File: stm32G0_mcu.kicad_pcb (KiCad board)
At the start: 4 copper layers, 70 x 45 mm, 54 parts, among them J1 Conn_01x04_Pin, J2 Conn_01x06_Pin, J3 Conn_01x04_Pin, SW1 SW_Nidec_CAS-120A1, SW2 SW_Push, SW3 SW_Push, U1 STM32G0B0KETx, U7 FT230XS

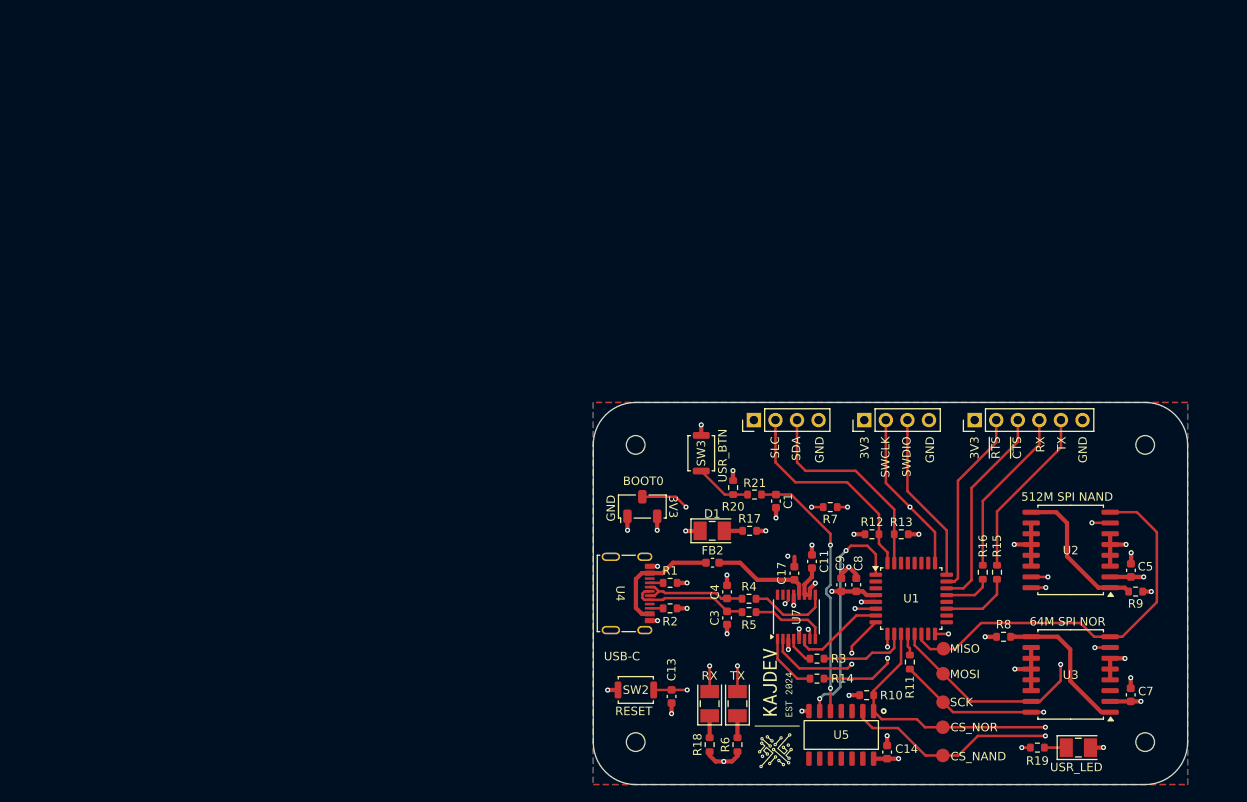
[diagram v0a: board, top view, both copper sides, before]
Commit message: fsdfsdf
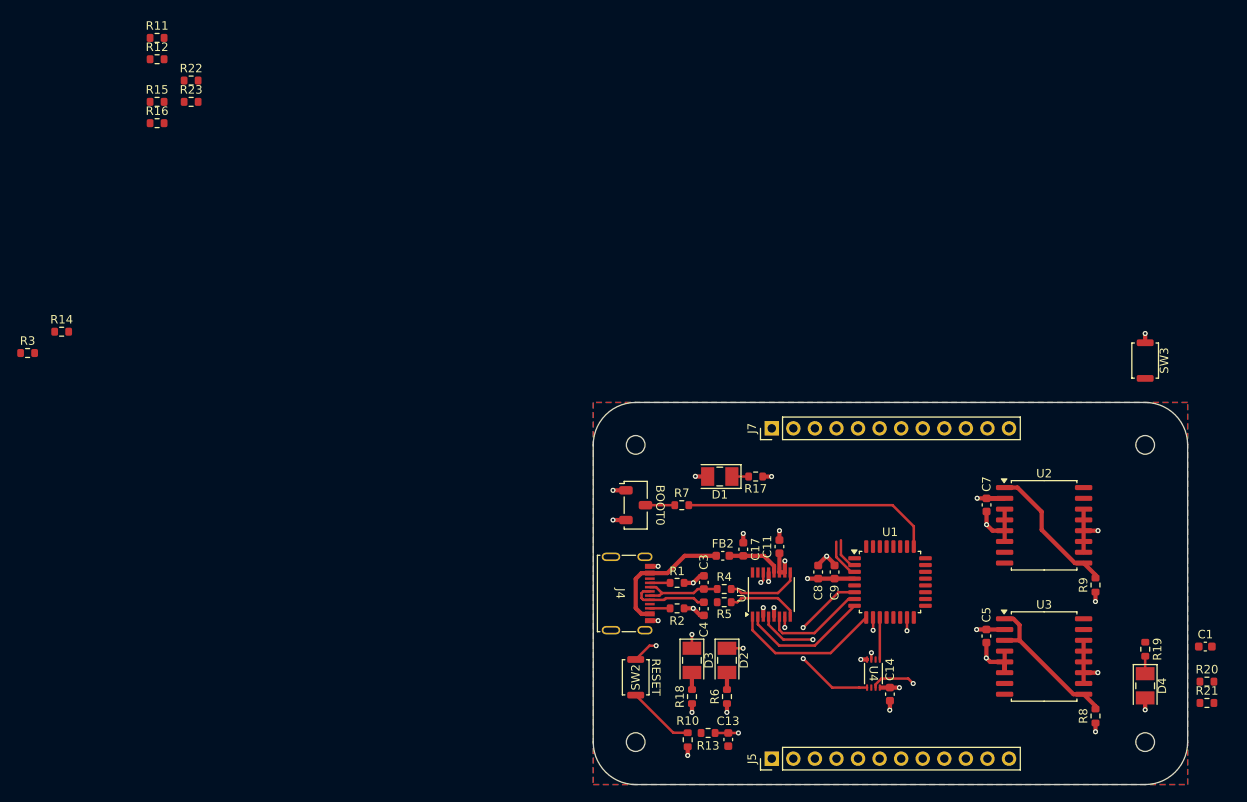
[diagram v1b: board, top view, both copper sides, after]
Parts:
- removed G***: LOGO, custom:logo
- removed J1, J3: Conn_01x04_Pin, Connector_PinHeader_2.54mm:PinHeader_1x04_P2.54mm_Vertical
- removed J2: Conn_01x06_Pin, Connector_PinHeader_2.54mm:PinHeader_1x06_P2.54mm_Vertical
- removed SW1: SW_Nidec_CAS-120A1, Button_Switch_SMD:Nidec_Copal_CAS-120A
- removed U5: ~, custom:74AC14SCX
- added BOOT0: SW_Nidec_CAS-120A1, Button_Switch_SMD:Nidec_Copal_CAS-120A, F.Cu at (105.0, 92.1)
- added J4: USB_C_Receptacle_USB2.0_16P, custom:640-USB4215-03-A, F.Cu at (102.7, 102.5)
- added J5: Conn_01x12_Pin, Connector_PinHeader_2.54mm:PinHeader_1x12_P2.54mm_Vertical, F.Cu at (121.0, 122.0)
- added J7: Conn_01x12_Pin, Connector_PinHeader_2.54mm:PinHeader_1x12_P2.54mm_Vertical, F.Cu at (121.0, 83.0)
- added R22: 1k8, Resistor_SMD:R_0603_1608Metric, F.Cu at (52.6, 42.1)
- added R23: 1k8, Resistor_SMD:R_0603_1608Metric, F.Cu at (52.6, 44.6)
- R10: value 56k -> 10k
- R12: value 1k8 -> 56k
- R13: value 1k8 -> 10k
- U4: footprint custom:640-USB4215-03-A -> custom:74HC3G14-Q100
- moved R11 115.2 mm to (48.6, 37.1), turned to 0 degrees
- moved R15 113.4 mm to (48.6, 44.6), turned to 0 degrees
- moved R16 110.7 mm to (48.6, 47.1), turned to 0 degrees
- moved R12 101.1 mm to (48.6, 39.6), turned to 0 degrees
- moved R3 99.7 mm to (33.4, 74.2)
- moved R14 97.9 mm to (37.4, 71.7), turned to 0 degrees
- moved H1 69.5 mm to (165.0, 120.0)
- moved R20 60.3 mm to (172.3, 112.9), turned to 0 degrees
- moved H3 60.0 mm to (105.0, 120.0)
- moved R21 58.7 mm to (172.3, 115.4)
- moved SW3 53.4 mm to (165.0, 75.1)
- moved C1 53.4 mm to (172.1, 108.8), turned to 0 degrees
- moved H4 35.0 mm to (105.0, 85.0)
- moved R13 32.6 mm to (113.5, 118.9)
- moved U4 31.8 mm to (133.0, 111.9), turned to 180 degrees
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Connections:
- C13 pad 2: NRST -> RST
- C3 pad 1: USB_D+ -> USB_D-
- C4 pad 1: USB_D- -> USB_D+
- D1 pad 1: +3.3V -> GND
- D1 pad 2: GND -> /POWER_SUPPLY/PWR_LED
- D2 pad 2: +3.3V -> /POWER_SUPPLY/TX_LED
- D3 pad 2: +3.3V -> /POWER_SUPPLY/RX_LED
- R10 pad 1: FLASH_CS -> RST
- R12 pad 1: I2C1_SCL -> FLASH_CS
- R13 pad 1: I2C1_SDA -> RST
- R13 pad 2: +3.3V -> RST
- R15 pad 2: UART1_TX -> Net-(J5-Pin_5)
- R16 pad 1: UART1_RX -> Net-(J5-Pin_4)
- R17 pad 2: +3.3V -> /POWER_SUPPLY/PWR_LED
- R18 pad 2: +3.3V -> /POWER_SUPPLY/RX_LED
- R20 pad 1: +3.3V -> Net-(R20-Pad1)
- R20 pad 2: ~{USER_BTN} -> +3.3V
- R21 pad 2: ~{USER_BTN} -> Net-(R20-Pad1)
- R5 pad 1: USB_D+ -> Net-(U7-USBDP)
- R6 pad 2: +3.3V -> /POWER_SUPPLY/TX_LED
- R8 pad 2: Net-(U3-HOLD(IO_{3})) -> Net-(U3-~{HOLD}(IO_{3}))
- SW2 pad 2: NRST -> RST
- SW3 pad 2: ~{USER_BTN} -> Net-(R20-Pad1)
- U1 pad 15: unconnected-(U1-PB0-Pad15) -> PB0
- U1 pad 17: unconnected-(U1-PB2-Pad17) -> PB2
- U1 pad 18: unconnected-(U1-PA8-Pad18) -> PA8
- U1 pad 2: unconnected-(U1-PC14-Pad2) -> PC14
- U1 pad 20: unconnected-(U1-PC6-Pad20) -> PC6
- U1 pad 26: unconnected-(U1-PA15-Pad26) -> PA15
- U1 pad 27: unconnected-(U1-PB3-Pad27) -> PB3
- U1 pad 28: unconnected-(U1-PB4-Pad28) -> PB4
- U1 pad 29: unconnected-(U1-PB5-Pad29) -> PB5
- U1 pad 3: unconnected-(U1-PC15-Pad3) -> PC15
- U1 pad 30: unconnected-(U1-PB6-Pad30) -> PB6
- U3 pad 1: Net-(U3-HOLD(IO_{3})) -> Net-(U3-~{HOLD}(IO_{3}))
- U3 pad 3: unconnected-(U3-RESET-Pad3) -> Net-(U3-~{HOLD}(IO_{3}))
- U3 pad 9: Net-(U3-HOLD(IO_{3})) -> Net-(U3-~{HOLD}(IO_{3}))
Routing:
- net FLASH_CS: track 61.2 -> 4.95 mm, vias 2 -> 0
- net SPI1_MISO: track 47.3 -> 0.00 mm
- net ~{USER_BTN}: track 37.9 -> 0.00 mm, vias 2 -> 0
- net SPI1_SCK: track 37.7 -> 0.00 mm, vias 2 -> 0
- net SPI1_MOSI: track 37.1 -> 0.00 mm, vias 2 -> 0
- net FLASH_NOR_CS: track 41.7 -> 5.34 mm, vias 2 -> 1
- net RST: track 0.00 -> 31.6 mm, vias 0 -> 2
- net UART1_TX: track 28.6 -> 0.00 mm
- net USER_BTN: track 27.4 -> 0.00 mm, vias 2 -> 0
- net UART1_RX: track 25.4 -> 0.00 mm
- net I2C1_SDA: track 25.0 -> 0.00 mm
- net I2C1_SCL: track 24.9 -> 0.00 mm
- net ~{UART1_CTS}: track 24.4 -> 0.00 mm
- net ~{UART1_RTS}: track 22.0 -> 0.00 mm
- net USER_LED: track 20.5 -> 0.00 mm, vias 2 -> 0
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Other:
- board text removed: "3V3"
- board text removed: "512M SPI NAND"
- board text removed: "64M SPI NOR"
- board text removed: "BOOT0"
- board text removed: "CS_NAND"
- board text removed: "CS_NOR"
- board text removed: "GND"
- board text removed: "MISO"
- board text removed: "MOSI"
- board text removed: "RX"
- board text removed: "SCK"
- board text removed: "SDA"
- board text removed: "SLC"
- board text removed: "SWCLK"
- board text removed: "SWDIO"
- board text removed: "TX"
- board text removed: "USB-C"
- board text removed: "USR_BTN"
- board text removed: "USR_LED"
- board text removed: "~{CTS}"
- board text removed: "~{RTS}"

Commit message: asdsad
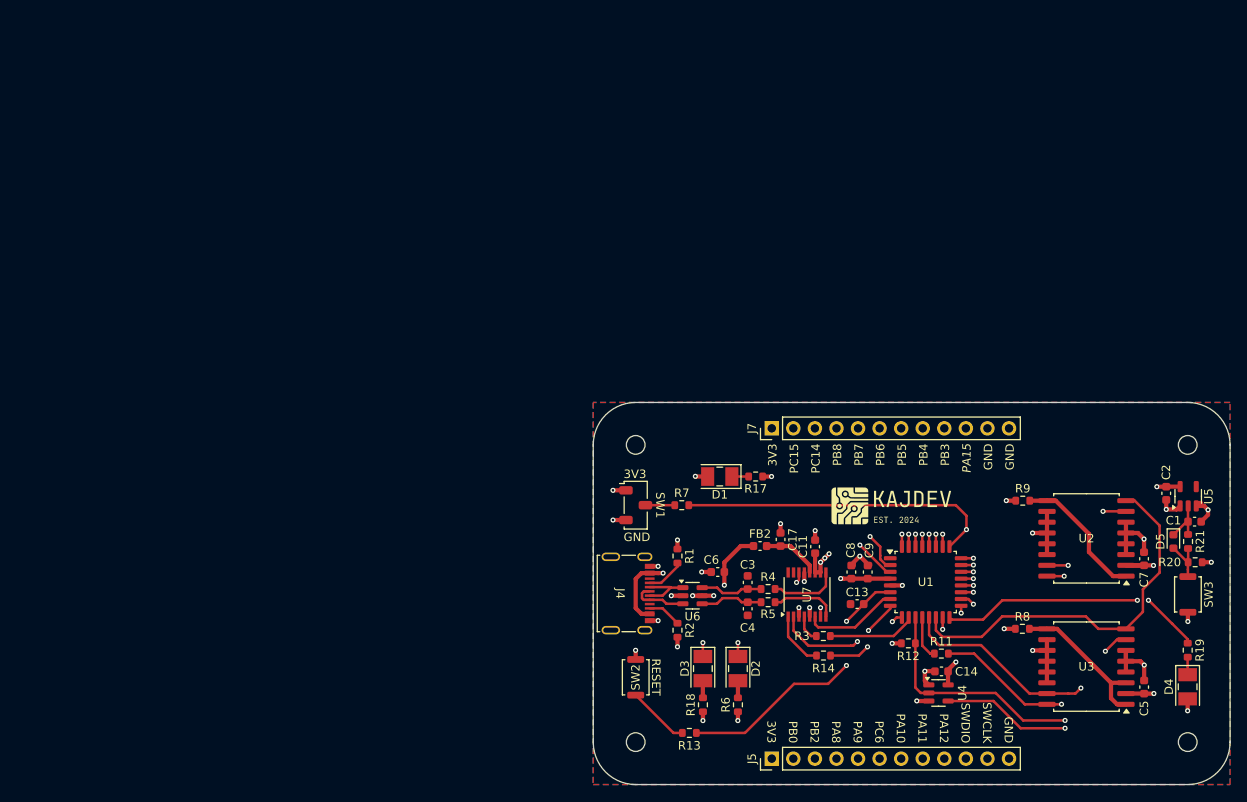
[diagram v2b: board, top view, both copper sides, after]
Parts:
- removed R10: 10k, Resistor_SMD:R_0603_1608Metric
- removed R15, R16: 120, Resistor_SMD:R_0603_1608Metric
- removed R22, R23: 1k8, Resistor_SMD:R_0603_1608Metric
- added C2: 100n, Capacitor_SMD:C_0603_1608Metric, F.Cu at (167.5, 90.7)
- added C6: 100n, Capacitor_SMD:C_0603_1608Metric, F.Cu at (114.7, 100.0)
- added D5: D, Diode_SMD:D_0603_1608Metric, F.Cu at (168.3, 96.4)
- added G***: LOGO, custom:logo2, F.Cu at (134.9, 92.2)
- added U5: SN74LVC1G14DBV, Package_TO_SOT_SMD:SOT-23-5, F.Cu at (170.1, 91.0)
- added U6: USBLC6-2SC6, Package_TO_SOT_SMD:SOT-23-6, F.Cu at (111.7, 102.8)
- U4: value ~ -> SN74LVC1G14DBV; footprint custom:74HC3G14-Q100 -> Package_TO_SOT_SMD:SOT-23-5
- moved R11 117.4 mm to (141.0, 109.6)
- moved R12 112.1 mm to (137.1, 108.4), turned to 180 degrees
- moved R3 99.5 mm to (127.1, 107.5)
- moved R14 97.5 mm to (127.1, 109.8)
- moved SW3 28.0 mm to (170.0, 102.6), turned to 90 degrees
- moved C13 22.0 mm to (131.1, 103.8), turned to 0 degrees
- moved C7 19.6 mm to (164.9, 98.4), turned to 90 degrees
- moved C5 19.5 mm to (164.9, 113.5), turned to 90 degrees
- moved R21 19.1 mm to (170.1, 96.4), turned to -90 degrees
- moved C1 14.8 mm to (170.8, 94.0)
- moved R20 14.1 mm to (170.9, 98.8)
- moved R8 13.4 mm to (150.5, 106.7), turned to 0 degrees
- moved R9 13.1 mm to (150.6, 91.6), turned to 0 degrees
- moved U4 7.99 mm to (140.7, 114.2), turned to 0 degrees
- moved C14 6.64 mm to (141.0, 111.7), turned to 180 degrees
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- renumbered BOOT0 to SW1
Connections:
- C1 pad 1: ~{USER_BTN} -> Net-(D5-K)
- C13 pad 2: RST -> NRST
- J5 pad 10: PB6 -> SWDIO
- J5 pad 11: GND -> BOOT0
- J5 pad 2: ~{UART1_RTS} -> PB0
- J5 pad 3: ~{UART1_CTS} -> PB2
- J5 pad 4: Net-(J5-Pin_4) -> PA8
- J5 pad 5: Net-(J5-Pin_5) -> PA9
- J5 pad 6: BOOT0 -> PC6
- J5 pad 7: SWDIO -> PA10
- J5 pad 8: PA8 -> PA11
- J5 pad 9: PA15 -> PA12
- J7 pad 10: PB4 -> PA15
- J7 pad 11: PB5 -> NRST_PIN
- J7 pad 2: I2C1_SDA -> PC15
- J7 pad 3: I2C1_SCL -> PC14
- J7 pad 4: PC6 -> PB8
- J7 pad 5: PC14 -> PB7
- J7 pad 6: PC15 -> PB6
- J7 pad 7: PB0 -> PB5
- J7 pad 8: PB2 -> PB4
- R13 pad 1: RST -> NRST
- R13 pad 2: RST -> NRST
- R21 pad 1: ~{USER_BTN} -> Net-(D5-K)
- R5 pad 1: Net-(U7-USBDP) -> USB_D+
- SW2 pad 2: RST -> NRST
- U1 pad 19: UART1_TX -> PA9
- U1 pad 21: UART1_RX -> PA10
- U1 pad 22: ~{UART1_CTS} -> PA11
- U1 pad 23: ~{UART1_RTS} -> PA12
- U1 pad 31: I2C1_SDA -> PB7
- U1 pad 32: I2C1_SCL -> PB8
- U4 pad 1: FLASH_CS -> GND
- U4 pad 2: USER_BTN -> FLASH_CS
- U4 pad 3: RST -> GND
- U4 pad 4: GND -> FLASH_NOR_CS
- U4 pad 5: NRST -> +3.3V
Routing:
- net FLASH_CS: track 4.95 -> 57.0 mm, vias 0 -> 2
- net BOOT0: track 33.4 -> 78.6 mm, vias 0 -> 1
- net SPI1_MISO: track 0.00 -> 44.8 mm
- net SPI1_MOSI: track 0.00 -> 40.6 mm, vias 0 -> 2
- net SPI1_SCK: track 0.00 -> 38.8 mm, vias 0 -> 2
- net SWDIO: track 0.00 -> 35.7 mm, vias 0 -> 1
- net PA12: track 0.00 -> 34.2 mm, vias 0 -> 1
- net PA11: track 0.00 -> 32.4 mm, vias 0 -> 1
- net PA10: track 0.00 -> 31.6 mm, vias 0 -> 1
- net RST: track 31.6 -> 0.00 mm, vias 2 -> 0
- net USER_LED: track 0.00 -> 31.5 mm, vias 0 -> 2
- net PC6: track 0.00 -> 30.2 mm, vias 0 -> 1
- net PA9: track 0.00 -> 29.5 mm, vias 0 -> 1
- net PA8: track 0.00 -> 28.3 mm, vias 0 -> 1
- net PB2: track 0.00 -> 27.0 mm, vias 0 -> 1
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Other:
- board size 70 x 45 mm -> 75 x 45 mm
- board text added: "3V3"
- board text added: "GND"
- board text added: "PA10"
- board text added: "PA11"
- board text added: "PA12"
- board text added: "PA15"
- board text added: "PA8"
- board text added: "PA9"
- board text added: "PB0"
- board text added: "PB2"
- board text added: "PB3"
- board text added: "PB4"
- board text added: "PB5"
- board text added: "PB6"
- board text added: "PB7"
- board text added: "PB8"
- board text added: "PC14"
- board text added: "PC15"
- board text added: "PC6"
- board text added: "SWCLK"
- board text added: "SWDIO"
